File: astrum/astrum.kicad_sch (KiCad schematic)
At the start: 27 parts, among them J1 USB_C_Receptacle_USB2.0_16P, J11 Screw_Terminal_01x02, J2 Micro_SD_Card, J3 Screw_Terminal_01x02, U1 STM32H523CEUx, U3 USBLC6-2SC6, U4 W25Q32JVSS, U8 DRV8871DDA, U9 DRV8871DDA, Y1 25 mHz

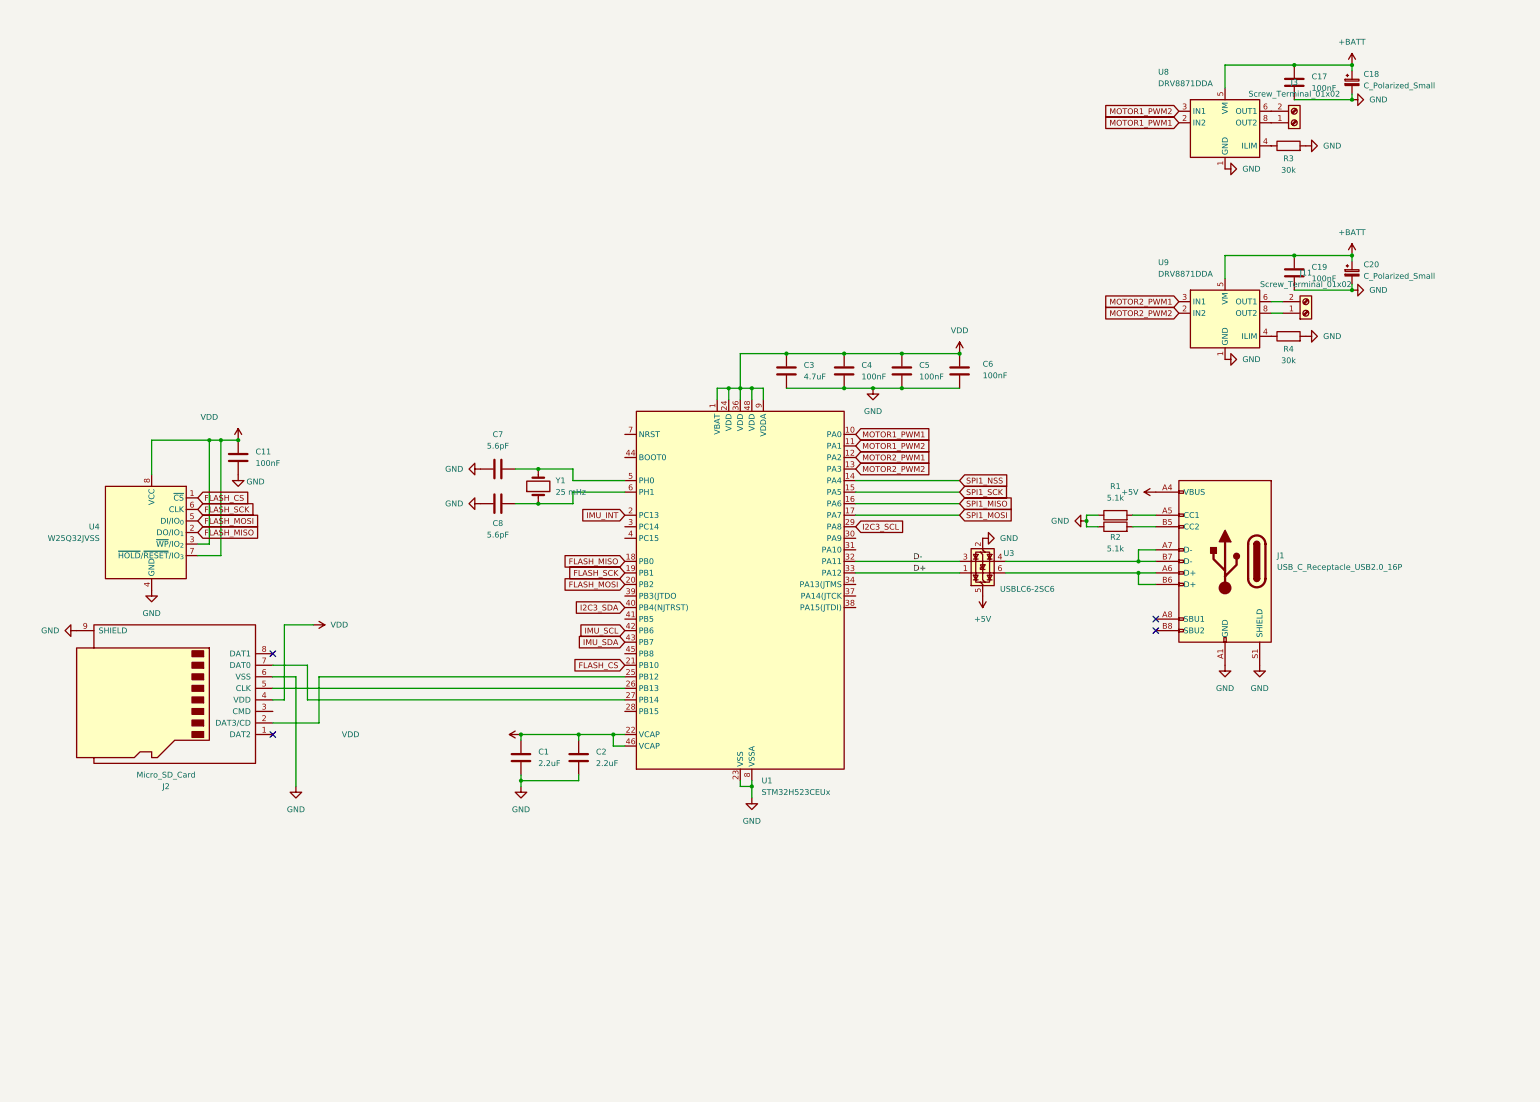
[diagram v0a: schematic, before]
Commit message: add imu schematics
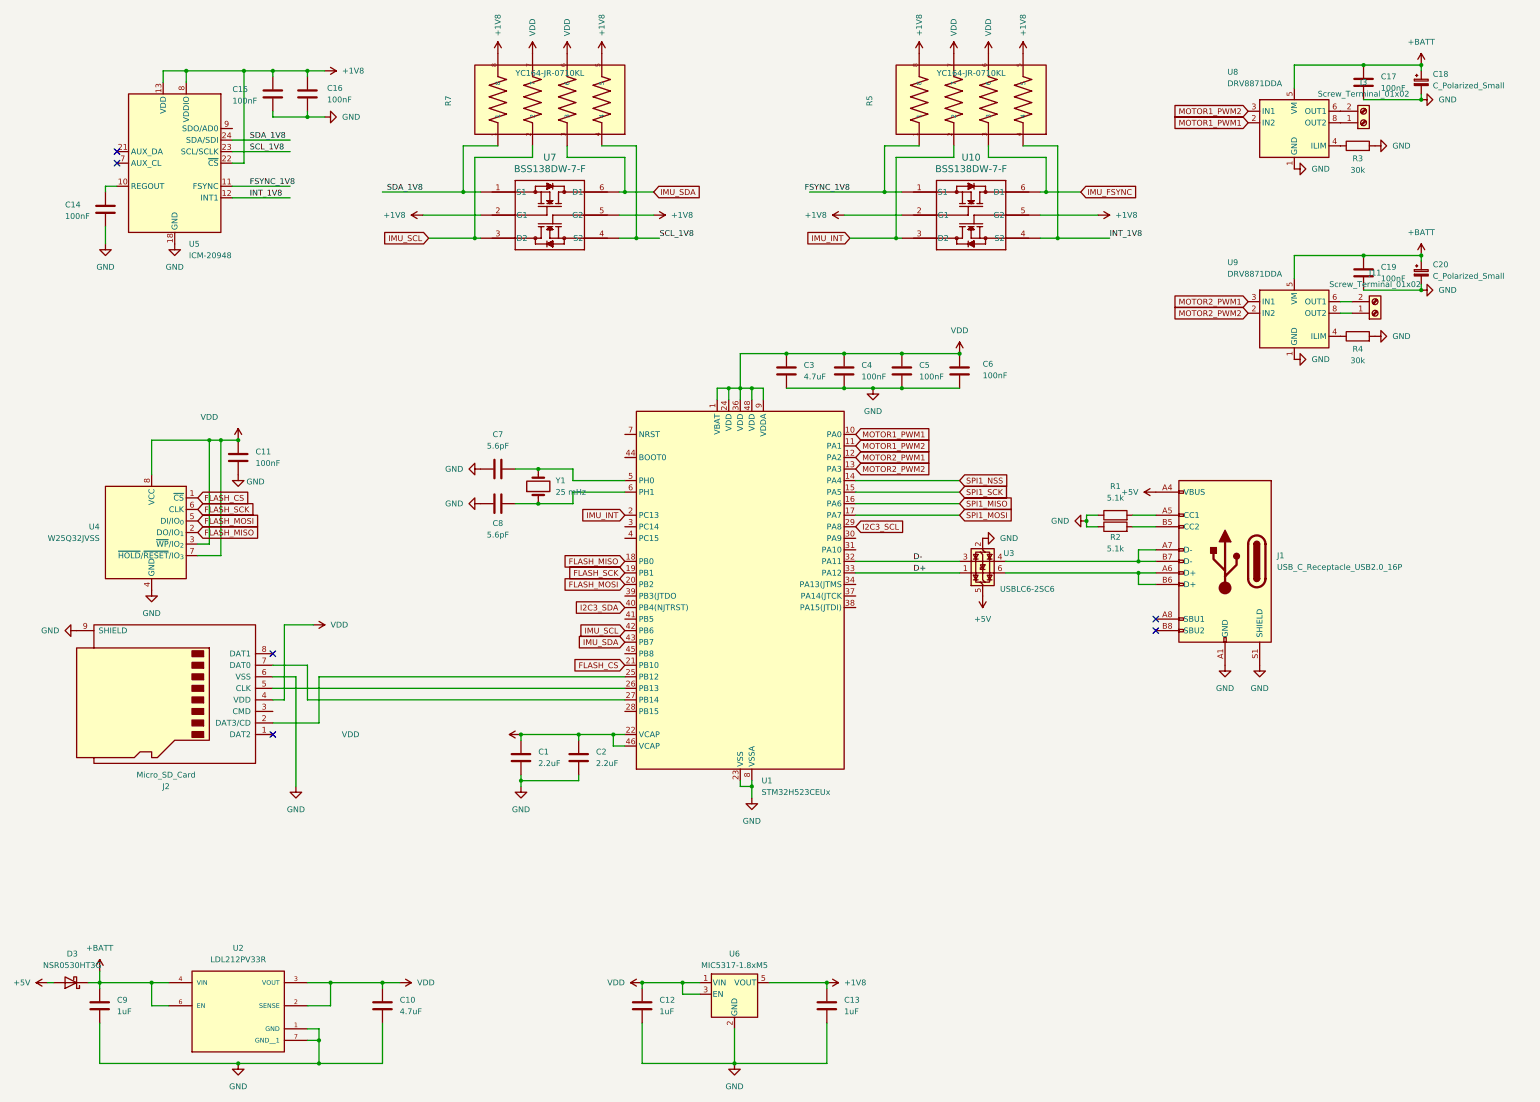
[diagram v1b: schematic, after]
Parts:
- added C10: 4.7uF, A_HDJ_Library:C_0603_1608Metric, symbol Device:C
- added C12, C13, C9: 1uF, A_HDJ_Library:C_0603_1608Metric, symbol Device:C
- added C14, C15, C16: 100nF, A_HDJ_Library:C_0603_1608Metric, symbol Device:C
- added D3: NSR0530HT3G, Diode_SMD:D_SOD-323, symbol Device:D_Schottky
- added R5, R7: YC164-JR-0710KL, YC164-JR-0710KL:RESCAXE80P320X160X70-8N, symbol YC164-JR-0710KL:YC164-JR-0710KL
- added U10, U7: BSS138DW-7-F, BSS138DW:SOT363_DIO, symbol 2025-10-04_02-12-38:BSS138DW-7-F
- added U2: LDL212PV33R, LDL212PV33R:SON50P200X200X80-7N, symbol LDL212PV33R:LDL212PV33R
- added U5: ICM-20948, Sensor_Motion:InvenSense_QFN-24_3x3mm_P0.4mm, symbol Sensor_Motion:ICM-20948
- added U6: MIC5317-1.8xM5, Package_TO_SOT_SMD:SOT-23-5, symbol Regulator_Linear:MIC5317-1.8xM5
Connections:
- net +5V: now also D3.2 (A)
- net +BATT: now also C9.1, D3.1 (K), U2.4 (VIN), U2.6 (EN)
- net GND: now also C10.2, C12.2, C13.2, C14.2, C15.2, C16.2, C9.2, U2.1 (GND), U2.7 (GND__1), U5.18 (GND), U5.20 (GND), U6.2 (GND)
- net IMU_INT: now also R5.2, U10.3 (D2)
- net IMU_SCL: now also R7.2, U7.3 (D2)
- net IMU_SDA: now also R7.3, U7.6 (D1)
- net VDD: now also C10.1, C12.1, R5.6, R5.7, R7.6, R7.7, U2.2 (SENSE), U2.3 (VOUT), U6.1 (VIN), U6.3 (EN)
- new net: C14.1, U5.10 (REGOUT)
- new net +1V8: C13.1, C15.1, C16.1, R5.5, R5.8, R7.5, R7.8, U10.2 (G1), U10.5 (G2), U5.13 (VDD), U5.22 (~{CS}), U5.8 (VDDIO), U6.5 (VOUT), U7.2 (G1), U7.5 (G2)
- new net FSYNC_1V8: R5.1, U10.1 (S1), U5.11 (FSYNC)
- new net IMU_FSYNC: R5.3, U10.6 (D1)
- new net INT_1V8: R5.4, U10.4 (S2), U5.12 (INT1)
- new net SCL_1V8: R7.4, U5.23 (SCL/SCLK), U7.4 (S2)
- new net SDA_1V8: R7.1, U5.24 (SDA/SDI), U7.1 (S1)
- no-connect marks 4 -> 6
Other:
- moved on the sheet: C17, C18, C19, C20, J11, J3, R3, R4, U8, U9
